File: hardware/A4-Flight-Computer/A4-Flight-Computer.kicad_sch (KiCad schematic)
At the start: 33 parts, among them J2 USB_C_Receptacle_USB2.0_14P, J3 LAB_Connector_02x20, J5 DEBUG, Q1 IRLML0030, SW1 RST, SW2 BOOT, U1 STM32H523RETx, U5 PTCAN3414DR

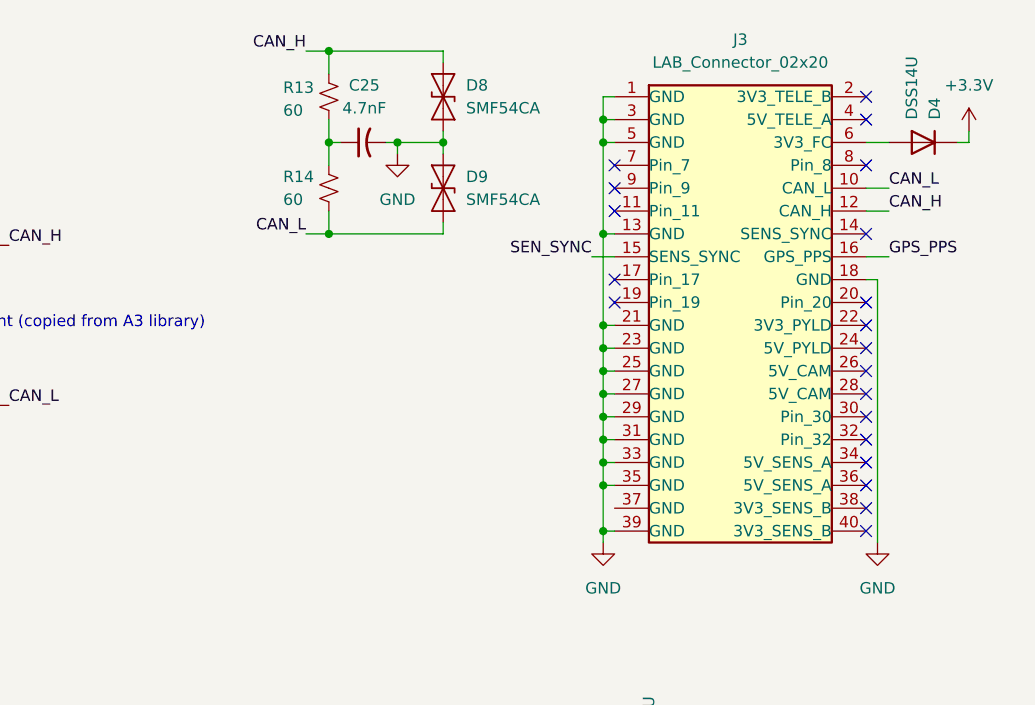
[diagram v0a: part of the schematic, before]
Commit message: update with new pcb standard revision
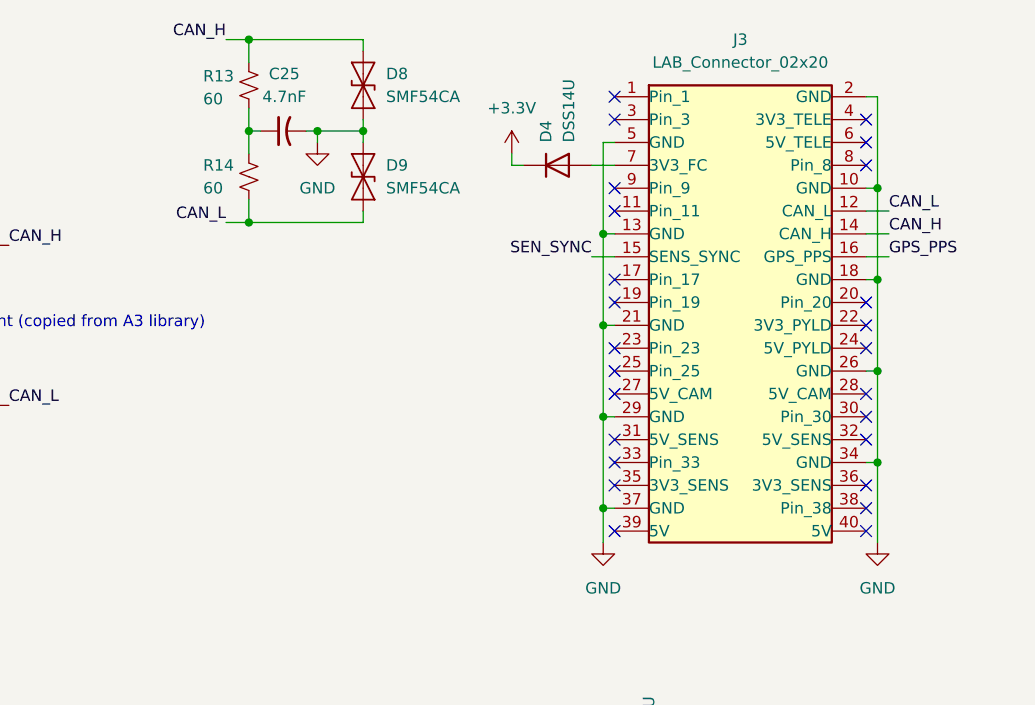
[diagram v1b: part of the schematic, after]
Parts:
- J3: footprint (none) -> LAB_PCB_Standard:LAB_PCB_With_Header
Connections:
- net CAN_H: now also J3.14 (CAN_H); no longer J3.12 (CAN_H)
- net CAN_L: now also J3.12 (CAN_L); no longer J3.10 (CAN_L)
- net GND: now also J3.10 (GND), J3.2 (GND), J3.26 (GND), J3.34 (GND), J3.37 (GND); no longer J3.1 (GND), J3.23 (GND), J3.25 (GND), J3.27 (GND), J3.3 (GND), J3.31 (GND), J3.33 (GND), J3.35 (GND), J3.39 (GND)
- net at J3.6 (5V_TELE): no longer D4.2 (A)
- net at J3.7 (3V3_FC): now also D4.2 (A)
- no-connect marks 55 -> 60
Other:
- moved on the sheet: C25, D4, D8, D9, R13, R14
